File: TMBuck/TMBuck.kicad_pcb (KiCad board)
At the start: 2 copper layers, 13 x 42.5 mm, 6 parts, among them J1 Pins, U1 LM2576S-5

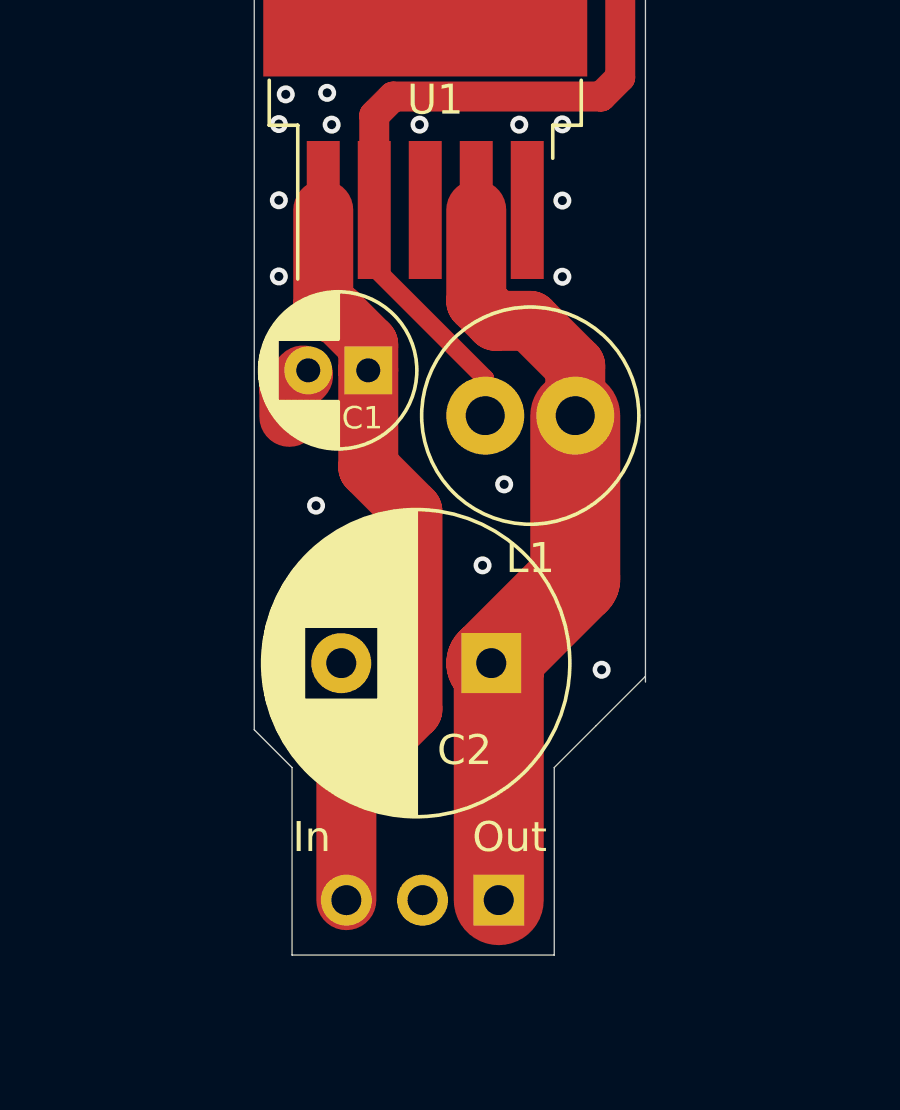
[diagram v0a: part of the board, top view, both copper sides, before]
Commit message: Inc Buck
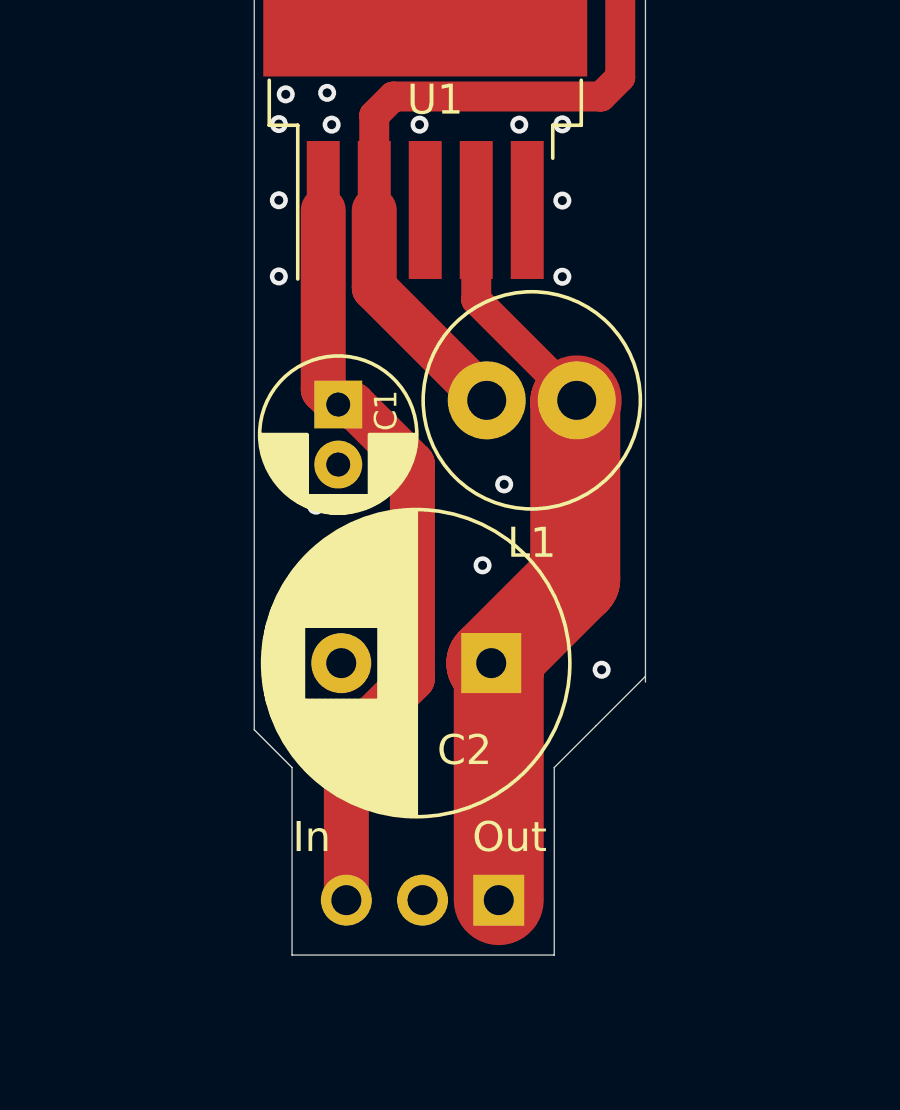
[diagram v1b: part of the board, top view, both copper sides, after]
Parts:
- moved C1 1.52 mm to (116.8, 90.7), turned to 270 degrees
- moved L1 0.51 mm to (124.7, 90.6)
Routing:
- net GND: track 1.57 -> 0.00 mm, vias 27 -> 26
- net Net-(D1-Pad1): track 34.1 -> 35.5 mm
- net +5V: track 26.3 -> 25.7 mm
